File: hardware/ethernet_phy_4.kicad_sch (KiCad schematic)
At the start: 29 parts, among them J3 RJMG1S8008101BR, SW2 SW TACT-SPST, U2 DP83826IRHBR, Y2 Crystal

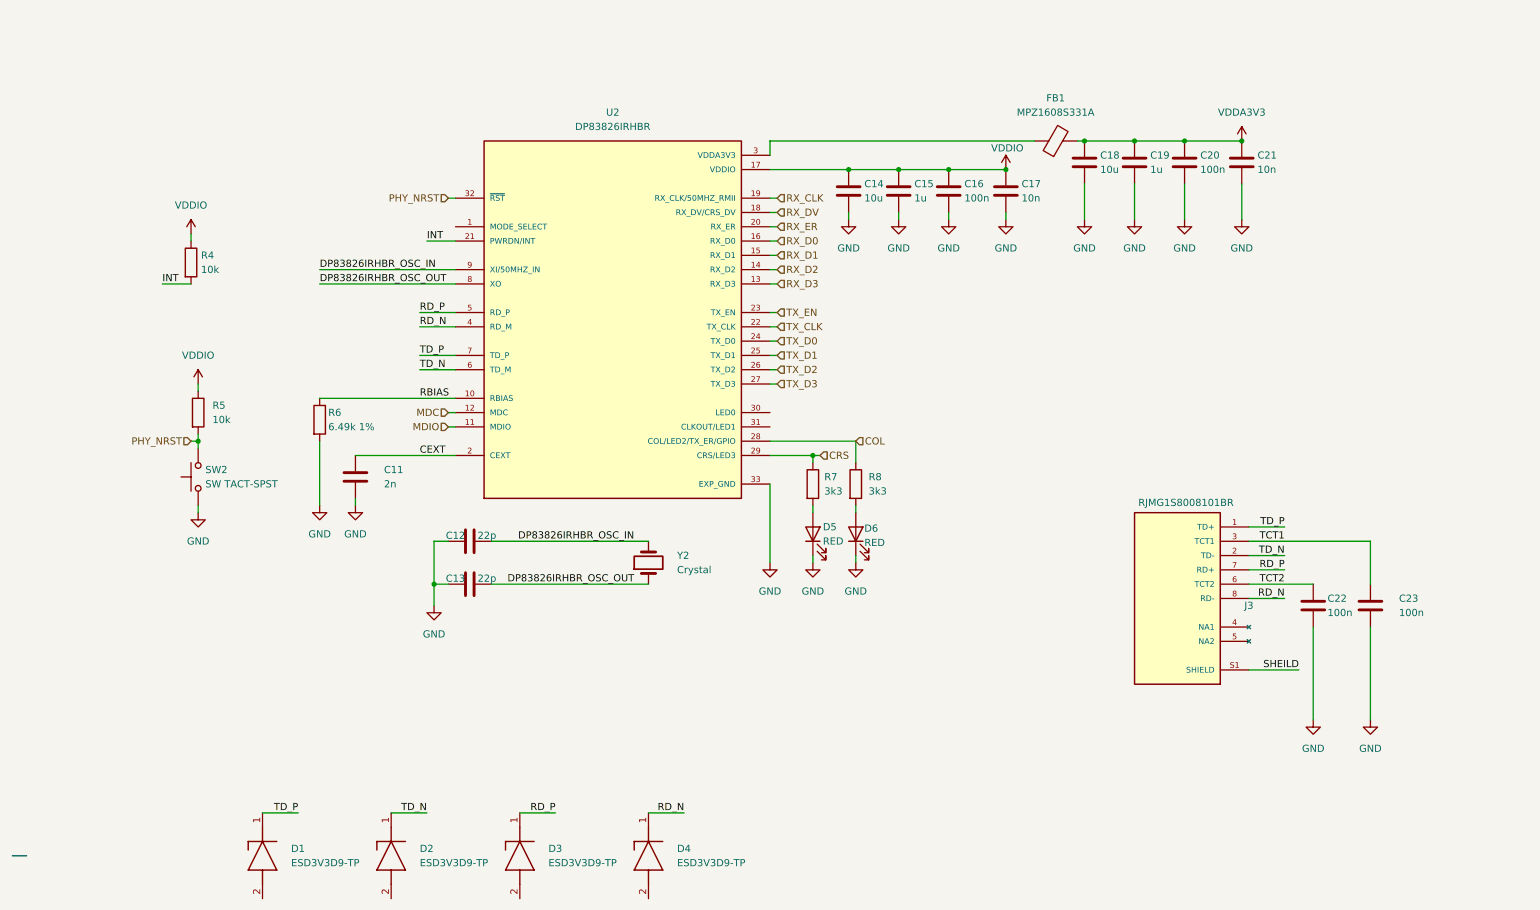
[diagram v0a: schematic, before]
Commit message: Organize schematic
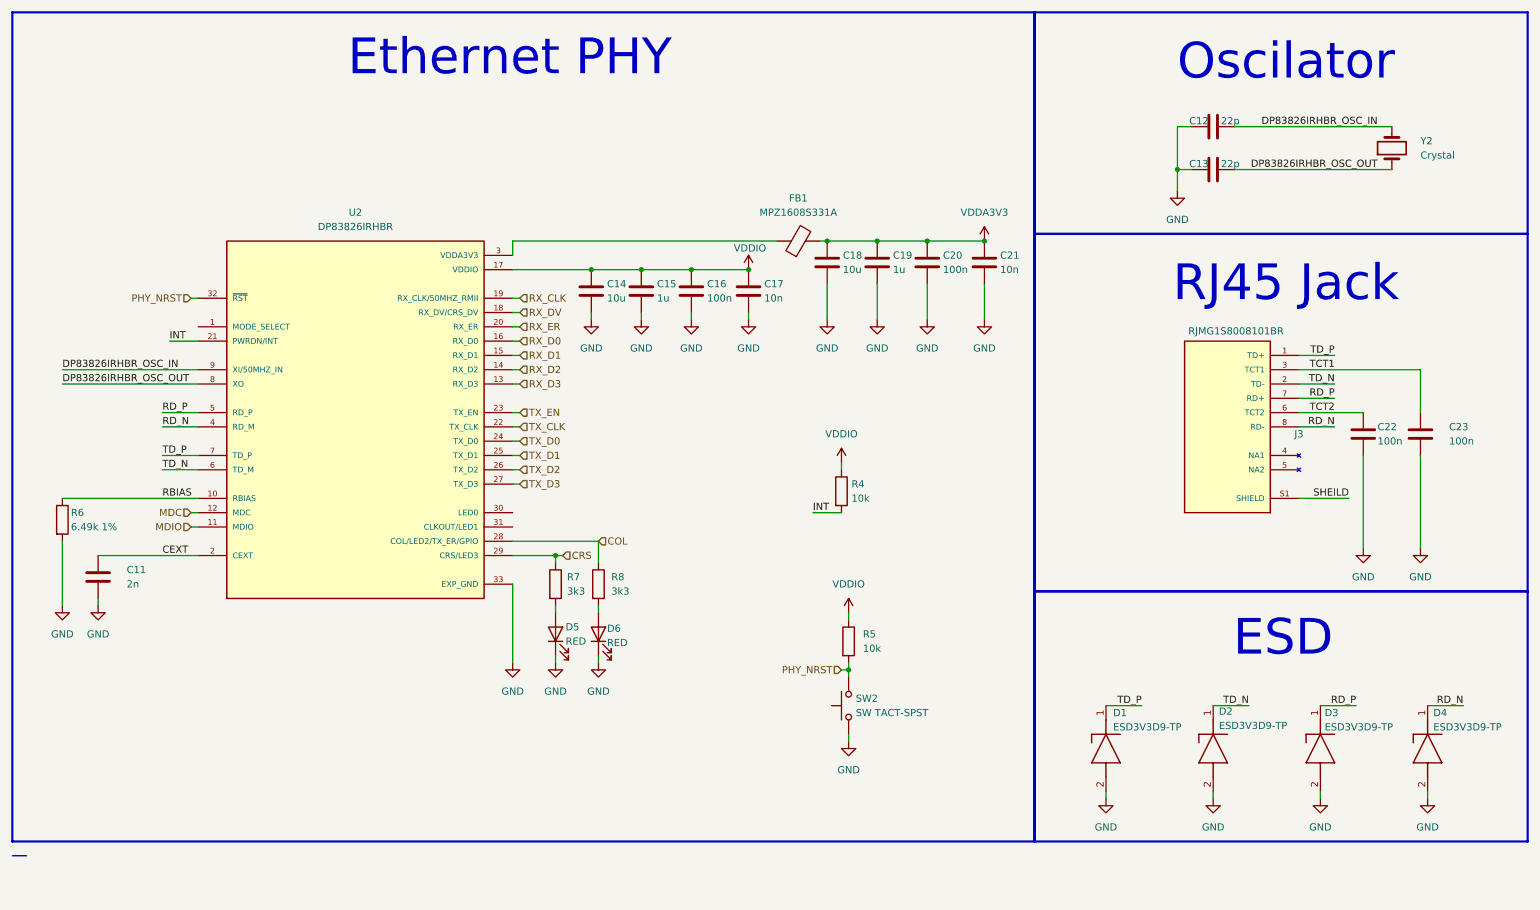
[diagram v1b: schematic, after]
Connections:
- net GND: now also D1.2 (A), D2.2 (A), D3.2 (A), D4.2 (A)
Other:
- note added: "ESD"
- note added: "Ethernet PHY"
- note added: "Oscilator"
- note added: "RJ45 Jack"
- moved on the sheet: C11, C12, C13, C14, C15, C16, C17, C18, C19, C20, C21, C22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
